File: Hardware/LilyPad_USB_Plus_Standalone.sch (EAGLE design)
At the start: 74 parts, among them J1 SEWTAP_LONG-2SIDE, J10 SEWTAP_LONG-2SIDE, J11 SEWTAP_LONG-2SIDE, J12 SEWTAP_LONG-2SIDE, J13 SEWTAP_LONG-2SIDE, J14 SEWTAP_LONG-2SIDE, J15 AMP FCI 10103594-0001LF, J2 SEWTAP_LONG-2SIDE, J3 SEWTAP_LONG-2SIDE, J4 SEWTAP_LONG-2SIDE, J5 SEWTAP_LONG-2SIDE, J6 SEWTAP_LONG-2SIDE, J7 SEWTAP_LONG-2SIDE, J8 SEWTAP_LONG-2SIDE, J9 SEWTAP_LONG-2SIDE, U1 MCP73831, U2 3.3V, U5 32U4, Y1 8MHz

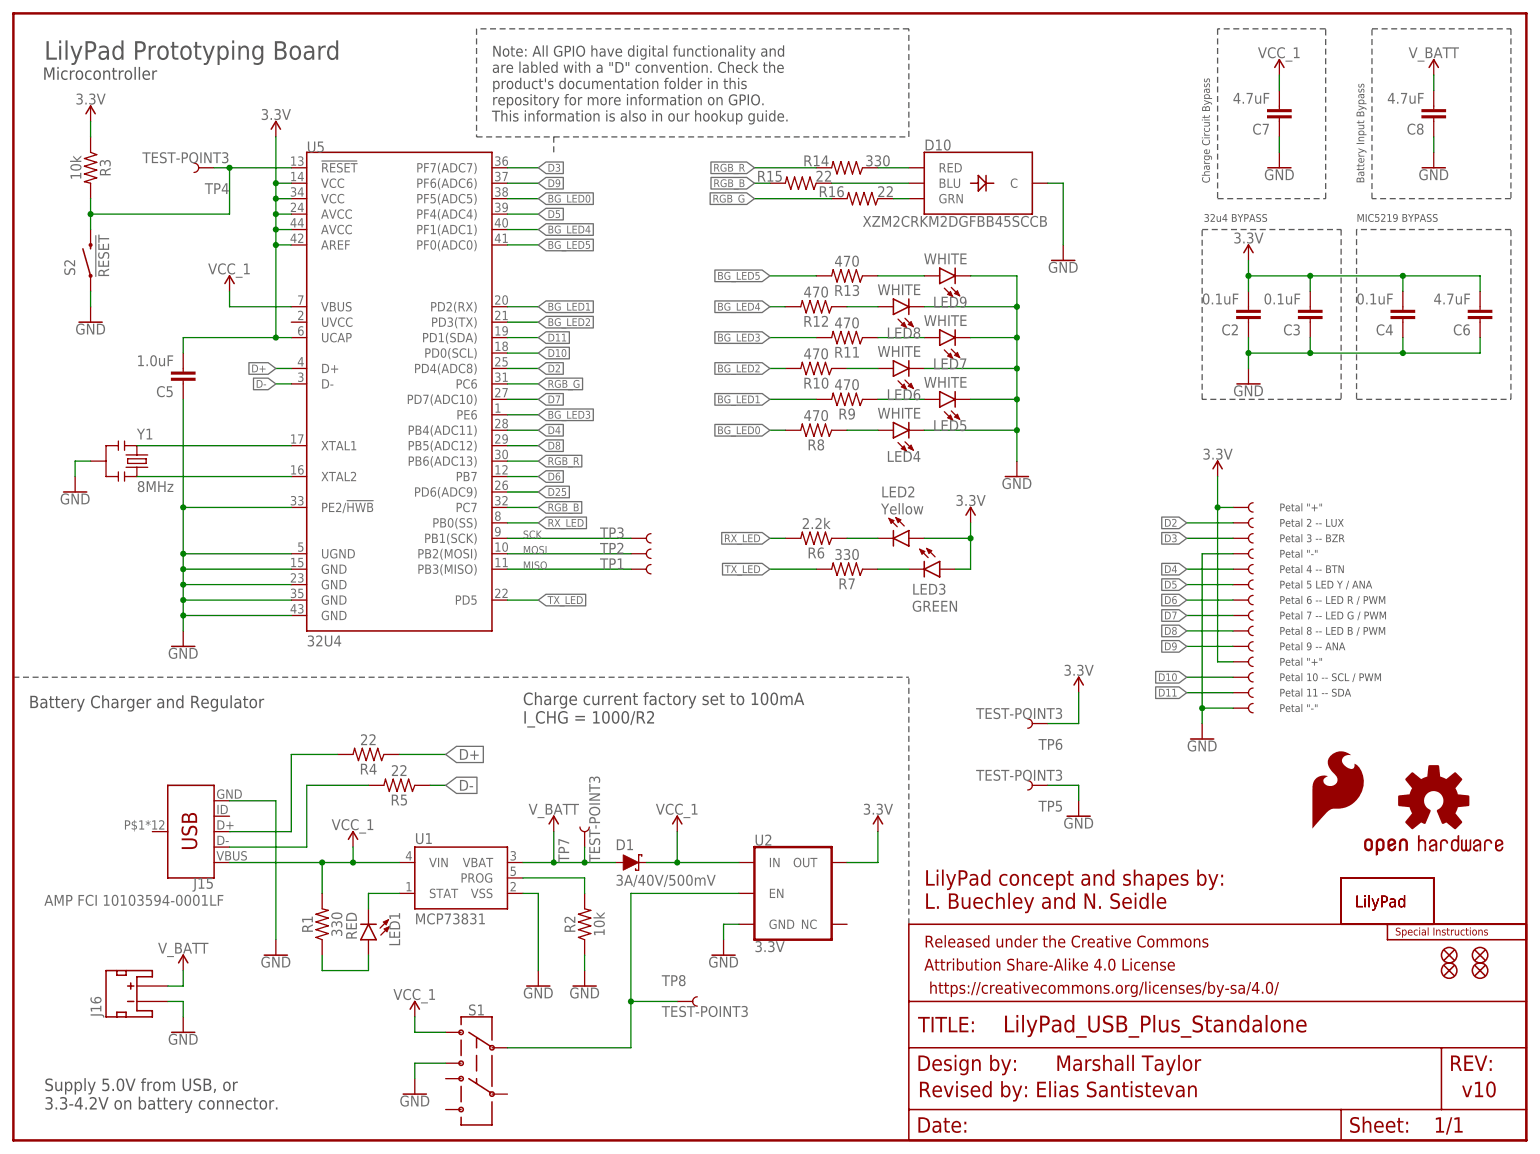
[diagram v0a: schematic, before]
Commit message: Changes after double check
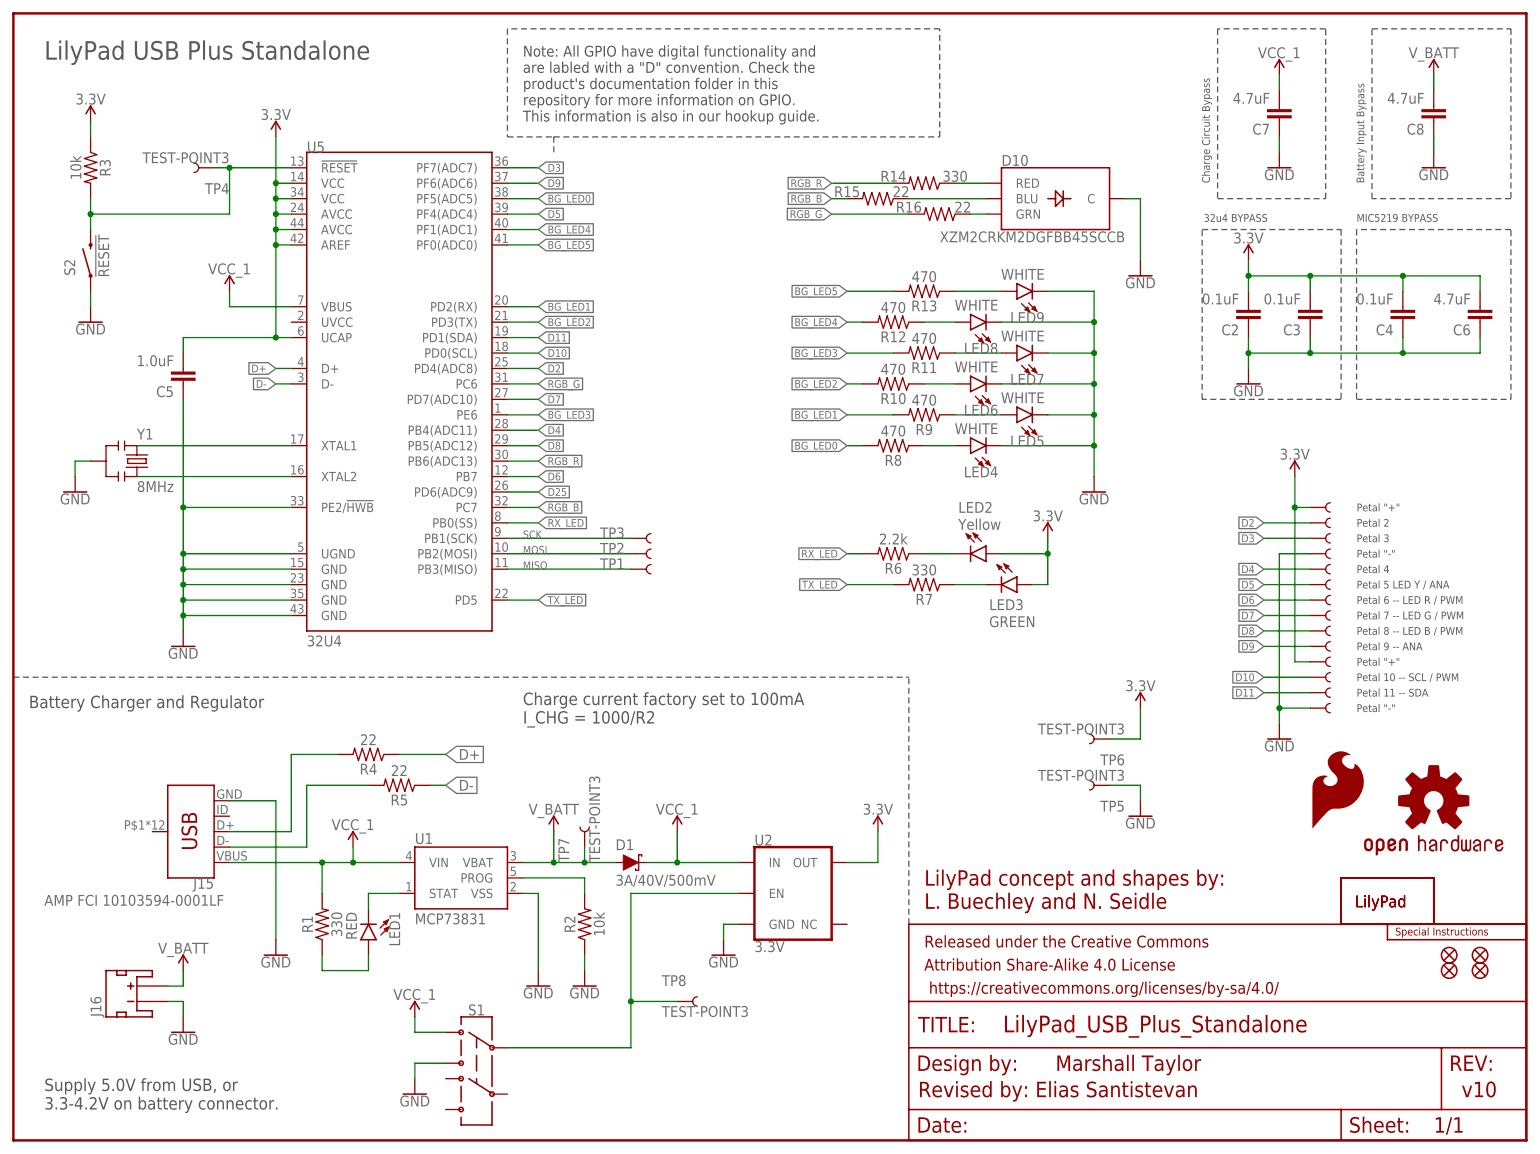
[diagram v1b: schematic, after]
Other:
- note added: "LilyPad USB Plus Standalone"
- note added: "Petal 2"
- note added: "Petal 3"
- note added: "Petal 4"
- note removed: "LilyPad Prototyping Board"
- note removed: "Microcontroller"
- note removed: "Petal 2 -- LUX"
- note removed: "Petal 3 -- BZR"
- note removed: "Petal 4 -- BTN"
- moved on the sheet: D10, LED2, LED3, LED4, LED5, LED6, LED7, LED8, LED9, R10, R11, R12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
